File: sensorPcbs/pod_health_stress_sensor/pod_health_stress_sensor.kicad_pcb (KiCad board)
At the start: 2 copper layers, 55.9 x 50.8 mm, 11 parts, among them J1 RJ45, J2 Screw_Terminal_1x08, U1 ADS1115

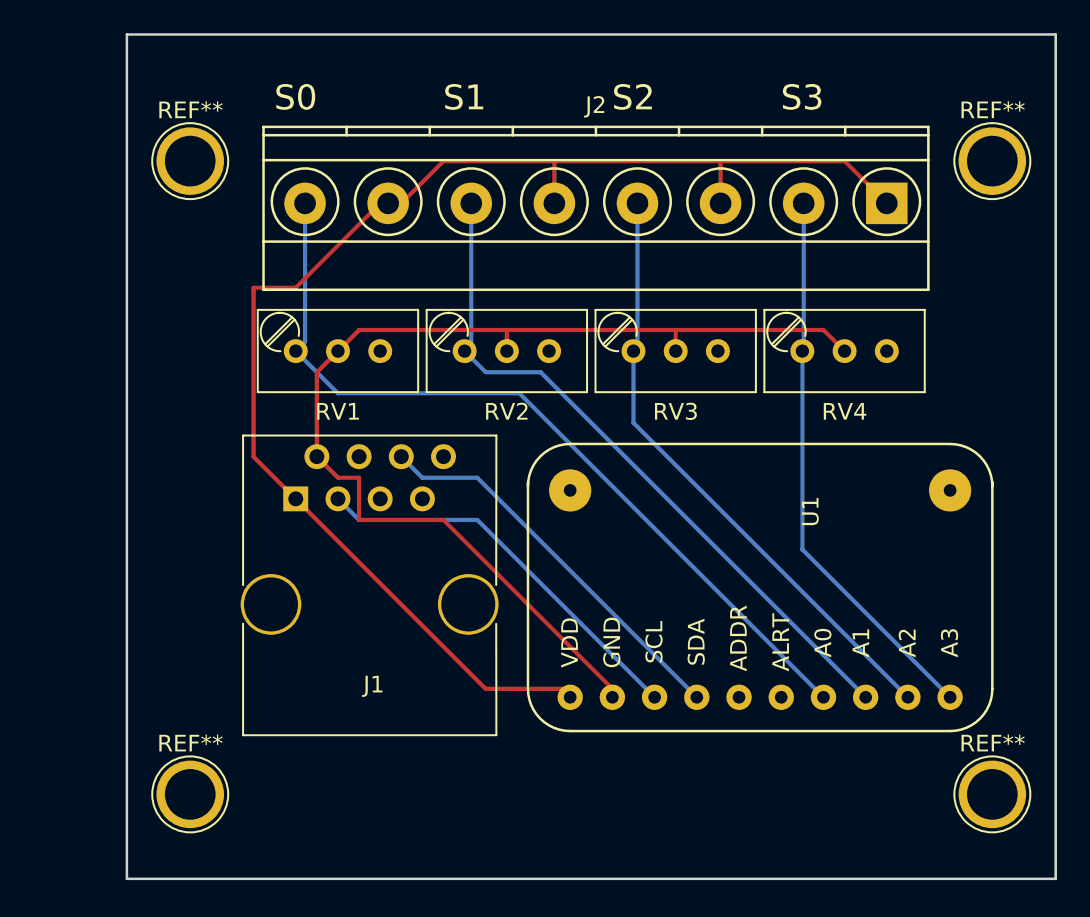
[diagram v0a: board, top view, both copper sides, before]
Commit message: added all the ferkin new ethernet shields to the sensor pcbs
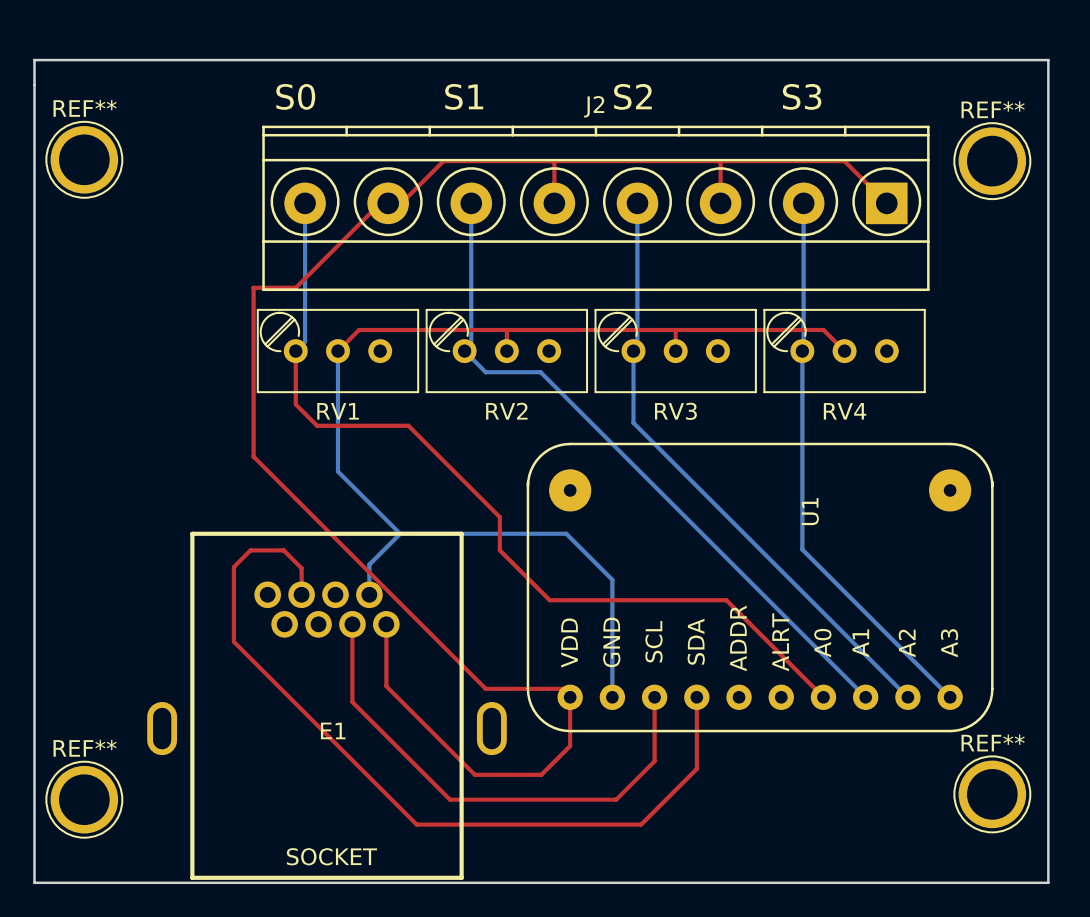
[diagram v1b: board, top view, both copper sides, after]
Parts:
- removed J1: RJ45, Connectors:RJ45_8
- added E1: RJE71-188-1401-ND, footprints:RJE71-188-1401-ND, F.Cu at (166.5, 91.0)
- moved REF** 6.38 mm to (160.0, 107.0)
- moved REF** 6.37 mm to (160.0, 68.5)
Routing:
- net SDA: track 24.3 -> 49.6 mm
- net 5V: track 83.1 -> 103.7 mm
- net SCL: track 24.0 -> 30.1 mm
- net GND: track 66.5 -> 72.5 mm
- net A0: track 49.5 -> 52.6 mm
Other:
- board size 55.9 x 50.8 mm -> 61 x 49.5 mm
